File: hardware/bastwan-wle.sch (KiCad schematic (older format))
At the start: 30 parts, among them J1 USB_B_Micro, J2 Conn_Right, J3 Conn_Left, J4 Conn_Battery, J5 SWD, Q1 DMG3415U-7, SW1 RST, U1 RAK3172, U2 AP2112K-3.3TRG1, U3 CP2102N-A01-GQFN28, U5 MCP73831-3-OT

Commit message: New_route
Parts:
- AE1: footprint Connectors:JST_S2B-PH-SM4-TB(LF)(SN) -> agroin:SMA_EDGE
- C1, C6: footprint (none) -> Capacitor_SMD:C_0402_1005Metric_Pad0.74x0.62mm_HandSolder
- J4: footprint bast-wan:JST_S2B-PH-SM4-TB(LF)(SN) -> Connectors:JST_S2B-PH-SM4-TB(LF)(SN)
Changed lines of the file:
@@
 F 0 "J4" V 3990 4570 50  0000 L CNN
 F 1 "Conn_Battery" H 3890 4370 50  0000 C CNN
-F 2 "bast-wan:JST_S2B-PH-SM4-TB(LF)(SN)" H 3840 4470 50  0001 C CNN
+F 2 "Connectors:JST_S2B-PH-SM4-TB(LF)(SN)" H 3840 4470 50  0001 C CNN
 F 3 "~" H 3840 4470 50  0001 C CNN
 F 4 "-" H -235 -70 50  0001 C CNN "manf#"
@@
 F 0 "AE1" H 7364 5719 50  0000 L CNN
 F 1 "Antenna" H 7364 5628 50  0000 L CNN
-F 2 "Connectors:JST_S2B-PH-SM4-TB(LF)(SN)" H 7220 5780 50  0001 C CNN
+F 2 "agroin:SMA_EDGE" H 7220 5780 50  0001 C CNN
 F 3 "~" H 7220 5780 50  0001 C CNN
 F 4 "-" H 1210 4435 50  0001 C CNN "manf#"
@@
 F 0 "C6" H 9392 2126 50  0000 L CNN
 F 1 "0.1uF" H 9392 2035 50  0000 L CNN
-F 2 "" H 9300 2080 50  0001 C CNN
+F 2 "Capacitor_SMD:C_0402_1005Metric_Pad0.74x0.62mm_HandSolder" H 9300 2080 50  0001 C CNN
 F 3 "~" H 9300 2080 50  0001 C CNN
 	1    9300 2080
@@
 F 0 "C1" H 5572 7311 50  0000 L CNN
 F 1 "0.1uF" H 5572 7220 50  0000 L CNN
-F 2 "" H 5480 7265 50  0001 C CNN
+F 2 "Capacitor_SMD:C_0402_1005Metric_Pad0.74x0.62mm_HandSolder" H 5480 7265 50  0001 C CNN
 F 3 "~" H 5480 7265 50  0001 C CNN
 	1    5480 7265

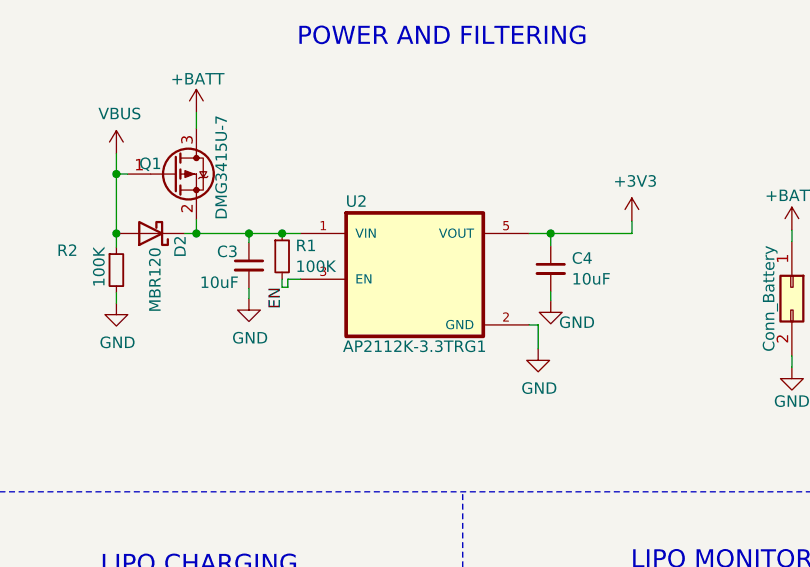
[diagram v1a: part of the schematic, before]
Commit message: Change_Sch
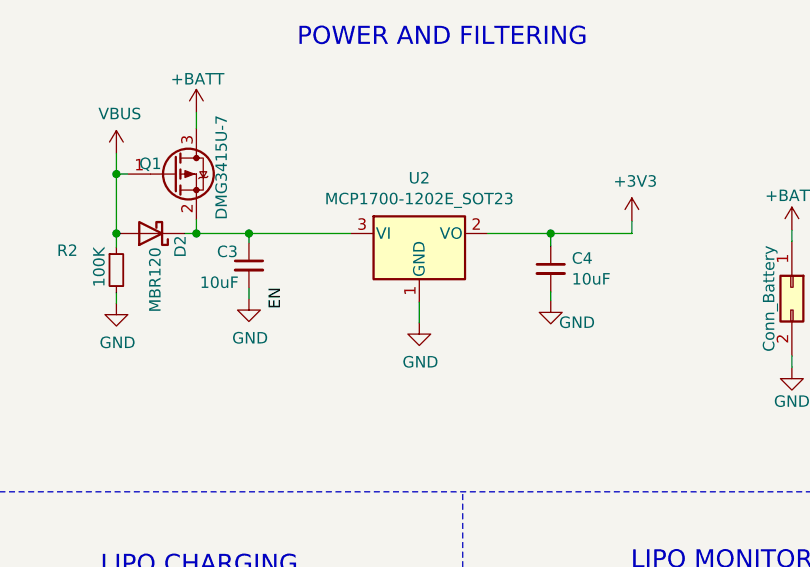
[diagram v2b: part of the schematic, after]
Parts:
- removed R1: 100K, Resistor_SMD:R_0402_1005Metric_Pad0.72x0.64mm_HandSolder, symbol Device:R_Small
- removed U2: AP2112K-3.3TRG1, Package_TO_SOT_SMD:TSOT-23-5, symbol bastwan-wle-rescue:AP2112K-3.3TRG1-electroniccats-Bast_WAN-rescue
- added U2: MCP1700-1202E_SOT23, Package_TO_SOT_SMD:SOT-23, symbol Regulator_Linear:MCP1700-1202E_SOT23
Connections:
- net +3V3: now also U2.2 (VO)
- net GND: now also U2.1 (GND)
- net at C3.1, D2.1 (K), Q1.2 (S): now also U2.3 (VI)
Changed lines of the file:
@@
 D-
-$Comp
-L bastwan-wle-rescue:AP2112K-3.3TRG1-electroniccats-Bast_WAN-rescue U2
-U 1 1 5DC7B9FC
-P 2190 4435
-F 0 "U2" H 1935 4775 50  0000 C CNN
-F 1 "AP2112K-3.3TRG1" H 2190 4140 50  0000 C CNN
-F 2 "Package_TO_SOT_SMD:TSOT-23-5" H 2190 4435 50  0001 L BNN
-F 3 "SOT-753 Diodes Inc." H 2190 4435 50  0001 L BNN
-F 4 "AP2112K-3.3TRG1" H -235 30  50  0001 C CNN "manf#"
-	1    2190 4435
-	1    0    0    -1
-$EndComp
 $Comp
 L Battery_Management:MCP73831-3-OT U5
@@
 	1235 4235 1235 4175
 Wire Wire Line
-	2690 4235 2785 4235
-Wire Wire Line
 	3140 4235 3140 4180
-Wire Wire Line
-	2690 4635 2730 4635
-Wire Wire Line
-	2730 4635 2730 4740
 $Comp
 L power:GND #PWR022
 U 1 1 5DCBABFE
-P 2730 4740
-F 0 "#PWR022" H 2730 4490 50  0001 C CNN
-F 1 "GND" H 2735 4567 50  0000 C CNN
-F 2 "" H 2730 4740 50  0001 C CNN
-F 3 "" H 2730 4740 50  0001 C CNN
-	1    2730 4740
+P 2210 4625
+F 0 "#PWR022" H 2210 4375 50  0001 C CNN
+F 1 "GND" H 2215 4452 50  0000 C CNN
+F 2 "" H 2210 4625 50  0001 C CNN
+F 3 "" H 2210 4625 50  0001 C CNN
+	1    2210 4625
 	1    0    0    -1
 $EndComp
@@
 Text Label 8145 4575 0    79   ~ 0
 D13
-$Comp
-L Device:R_Small R1
-U 1 1 5DEE52DA
-P 1610 4335
-F 0 "R1" H 1669 4381 50  0000 L CNN
-F 1 "100K" H 1669 4290 50  0000 L CNN
-F 2 "Resistor_SMD:R_0402_1005Metric_Pad0.72x0.64mm_HandSolder" H 1610 4335 50  0001 C CNN
-F 3 "~" H 1610 4335 50  0001 C CNN
-F 4 "RC0603FR-07100KL" H -235 30  50  0001 C CNN "manf#"
-	1    1610 4335
-	1    0    0    -1
-$EndComp
-Wire Wire Line
-	1465 4235 1610 4235
-Connection ~ 1610 4235
-Wire Wire Line
-	1610 4235 1690 4235
-Wire Wire Line
-	1635 4435 1635 4470
-Wire Wire Line
-	1635 4470 1610 4470
-Wire Wire Line
-	1610 4470 1610 4435
-Wire Wire Line
-	1635 4435 1690 4435
 Text Label 1620 4470 3    50   ~ 0
 EN
@@
 Wire Notes Line
 	4935 8055 4920 8055
+$Comp
+L Regulator_Linear:MCP1700-1202E_SOT23 U2
+U 1 1 60F17AD5
+P 2210 4235
+F 0 "U2" H 2210 4477 50  0000 C CNN
+F 1 "MCP1700-1202E_SOT23" H 2210 4386 50  0000 C CNN
+F 2 "Package_TO_SOT_SMD:SOT-23" H 2210 4460 50  0001 C CNN
+F 3 "http://ww1.microchip.com/downloads/en/DeviceDoc/20001826D.pdf" H 2210 4235 50  0001 C CNN
+	1    2210 4235
+	1    0    0    -1
+$EndComp
+Wire Wire Line
+	2210 4535 2210 4625
+Wire Wire Line
+	2510 4235 2785 4235
+Wire Wire Line
+	1465 4235 1910 4235
 $EndSCHEMATC
